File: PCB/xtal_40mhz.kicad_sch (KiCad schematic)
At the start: 3 parts, among them Y1 40MHz

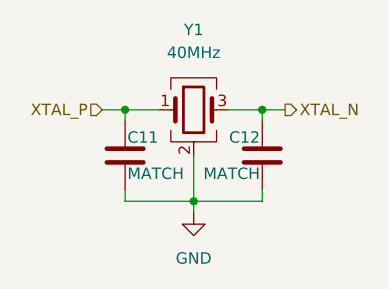
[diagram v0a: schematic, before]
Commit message: big things are happening
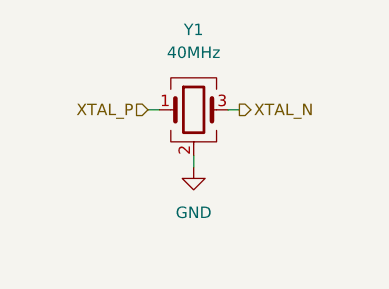
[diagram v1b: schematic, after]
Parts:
- removed C11, C12: MATCH, Capacitor_SMD:C_0603_1608Metric, symbol Device:C
- Y1: footprint (none) -> Crystal:Crystal_SMD_3225-4Pin_3.2x2.5mm
